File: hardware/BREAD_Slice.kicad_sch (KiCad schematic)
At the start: 16 parts, among them J10 Screw_Terminal_01x02, J11 Screw_Terminal_01x02, J12 Screw_Terminal_01x02, J13 Screw_Terminal_01x02, J14 Screw_Terminal_01x02, J15 Screw_Terminal_01x02, J16 Screw_Terminal_01x02, J2 Screw_Terminal_01x02, J3 Screw_Terminal_01x02, J4 Screw_Terminal_01x02, J5 Screw_Terminal_01x02, J6 Screw_Terminal_01x02, J7 Screw_Terminal_01x02, J8 Screw_Terminal_01x02, J9 Screw_Terminal_01x02, SW3 SW_SPDT

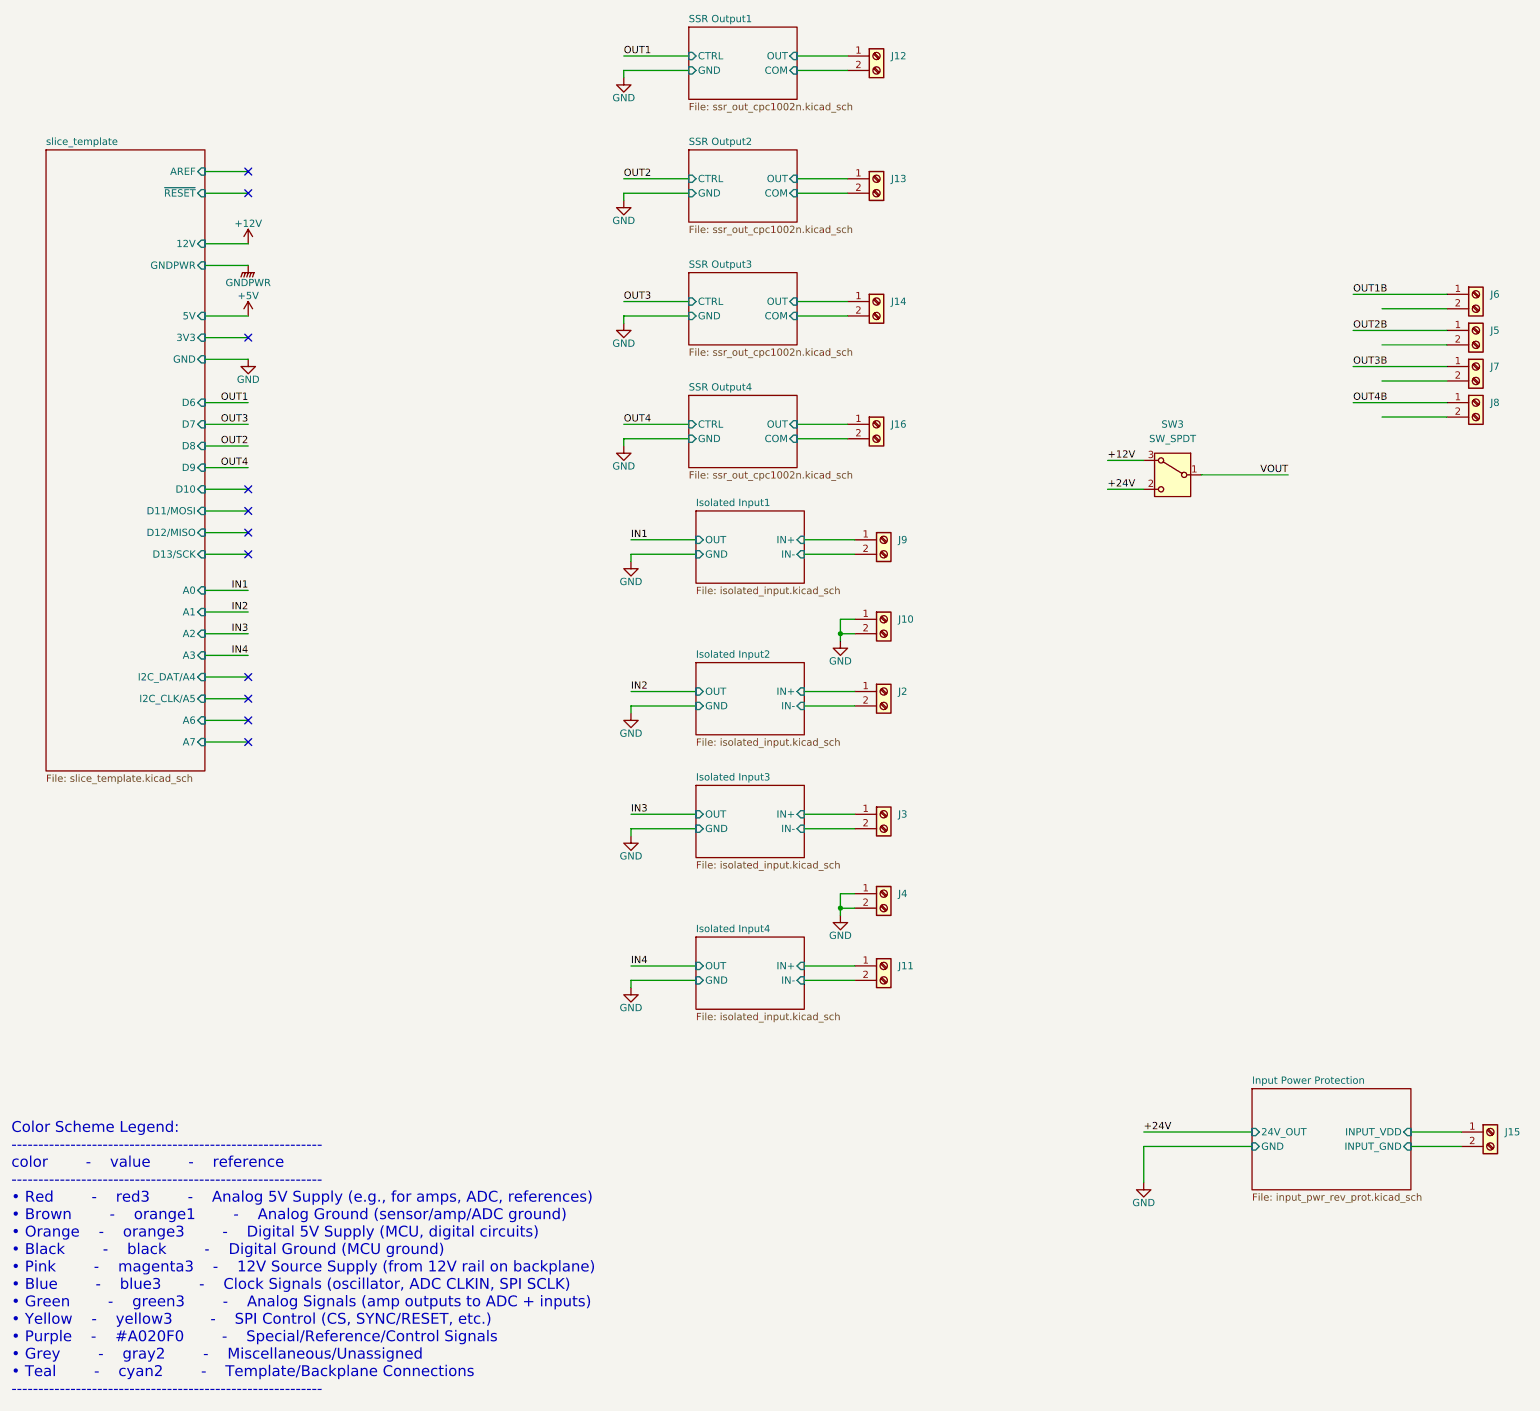
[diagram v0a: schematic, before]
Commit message: update schem
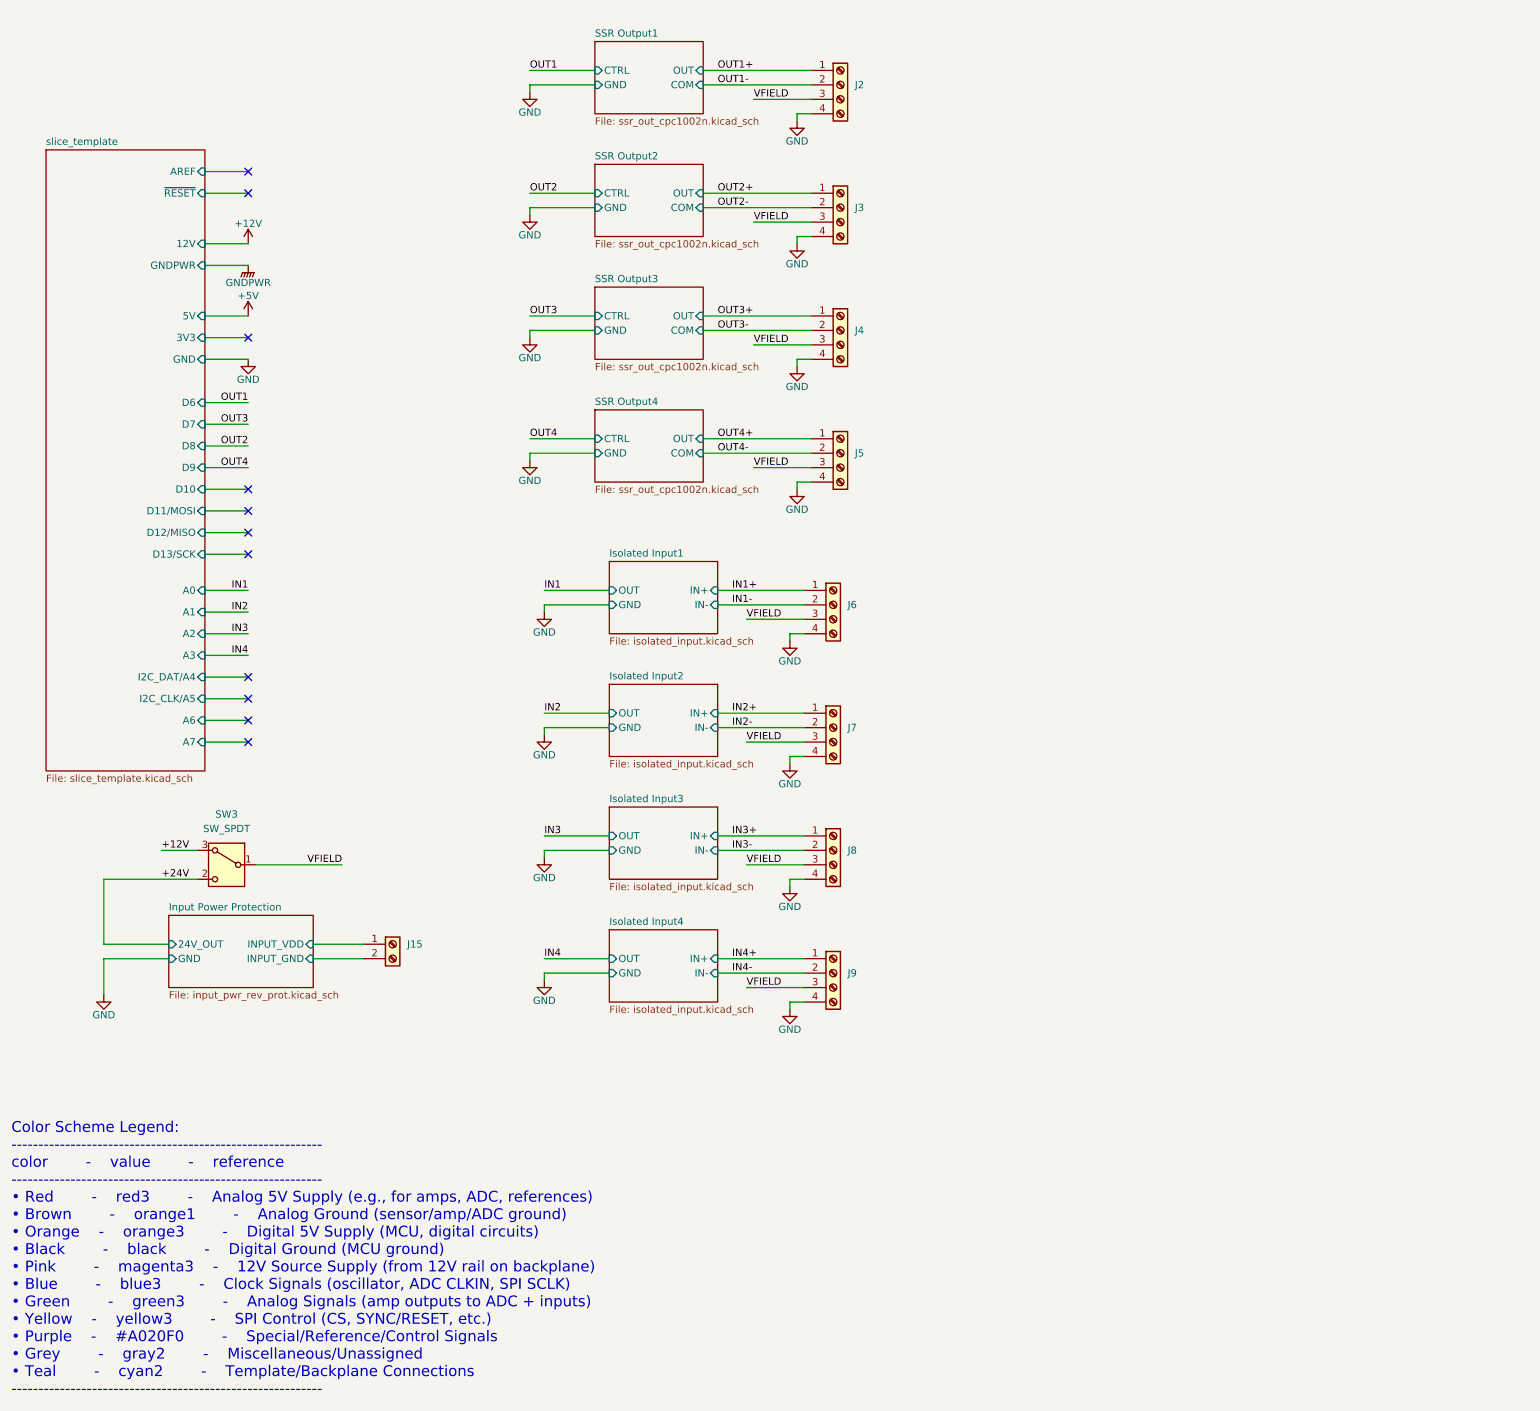
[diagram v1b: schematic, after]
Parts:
- removed J10, J11, J12, J13, J14, J16, J2, J3, J4, J5, J6, J7, J8, J9: Screw_Terminal_01x02, symbol Connector:Screw_Terminal_01x02
- added J2, J3, J4, J5, J6, J7, J8, J9: Screw_Terminal_01x04, symbol Connector:Screw_Terminal_01x04
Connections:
- net GND: now also J2.4 (Pin_4), J3.4 (Pin_4), J4.4 (Pin_4), J5.4 (Pin_4), J6.4 (Pin_4), J7.4 (Pin_4), J8.4 (Pin_4), J9.4 (Pin_4)
- net VOUT renamed VFIELD
- net VFIELD: now also J2.3 (Pin_3), J3.3 (Pin_3), J4.3 (Pin_3), J5.3 (Pin_3), J6.3 (Pin_3), J7.3 (Pin_3), J8.3 (Pin_3), J9.3 (Pin_3)
- new net IN1+: J6.1 (Pin_1)
- new net IN1-: J6.2 (Pin_2)
- new net IN2+: J7.1 (Pin_1)
- new net IN2-: J7.2 (Pin_2)
- new net IN3+: J8.1 (Pin_1)
- new net IN3-: J8.2 (Pin_2)
- new net IN4+: J9.1 (Pin_1)
- new net IN4-: J9.2 (Pin_2)
- new net OUT1+: J2.1 (Pin_1)
- new net OUT1-: J2.2 (Pin_2)
- new net OUT2+: J3.1 (Pin_1)
- new net OUT2-: J3.2 (Pin_2)
- new net OUT3+: J4.1 (Pin_1)
- new net OUT3-: J4.2 (Pin_2)
- new net OUT4+: J5.1 (Pin_1)
- new net OUT4-: J5.2 (Pin_2)
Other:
- moved on the sheet: J15, SW3
